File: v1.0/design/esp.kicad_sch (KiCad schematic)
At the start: 28 parts, among them J1 12402012E212A, J2 5v INPUT, J3 Conn_01x10, J4 Conn_01x10, SW1 PTS636_SM43_SMTR_LFS, SW2 PTS636_SM43_SMTR_LFS, U1 AMS1117-3.3, U1 ESP32-WROOM-E

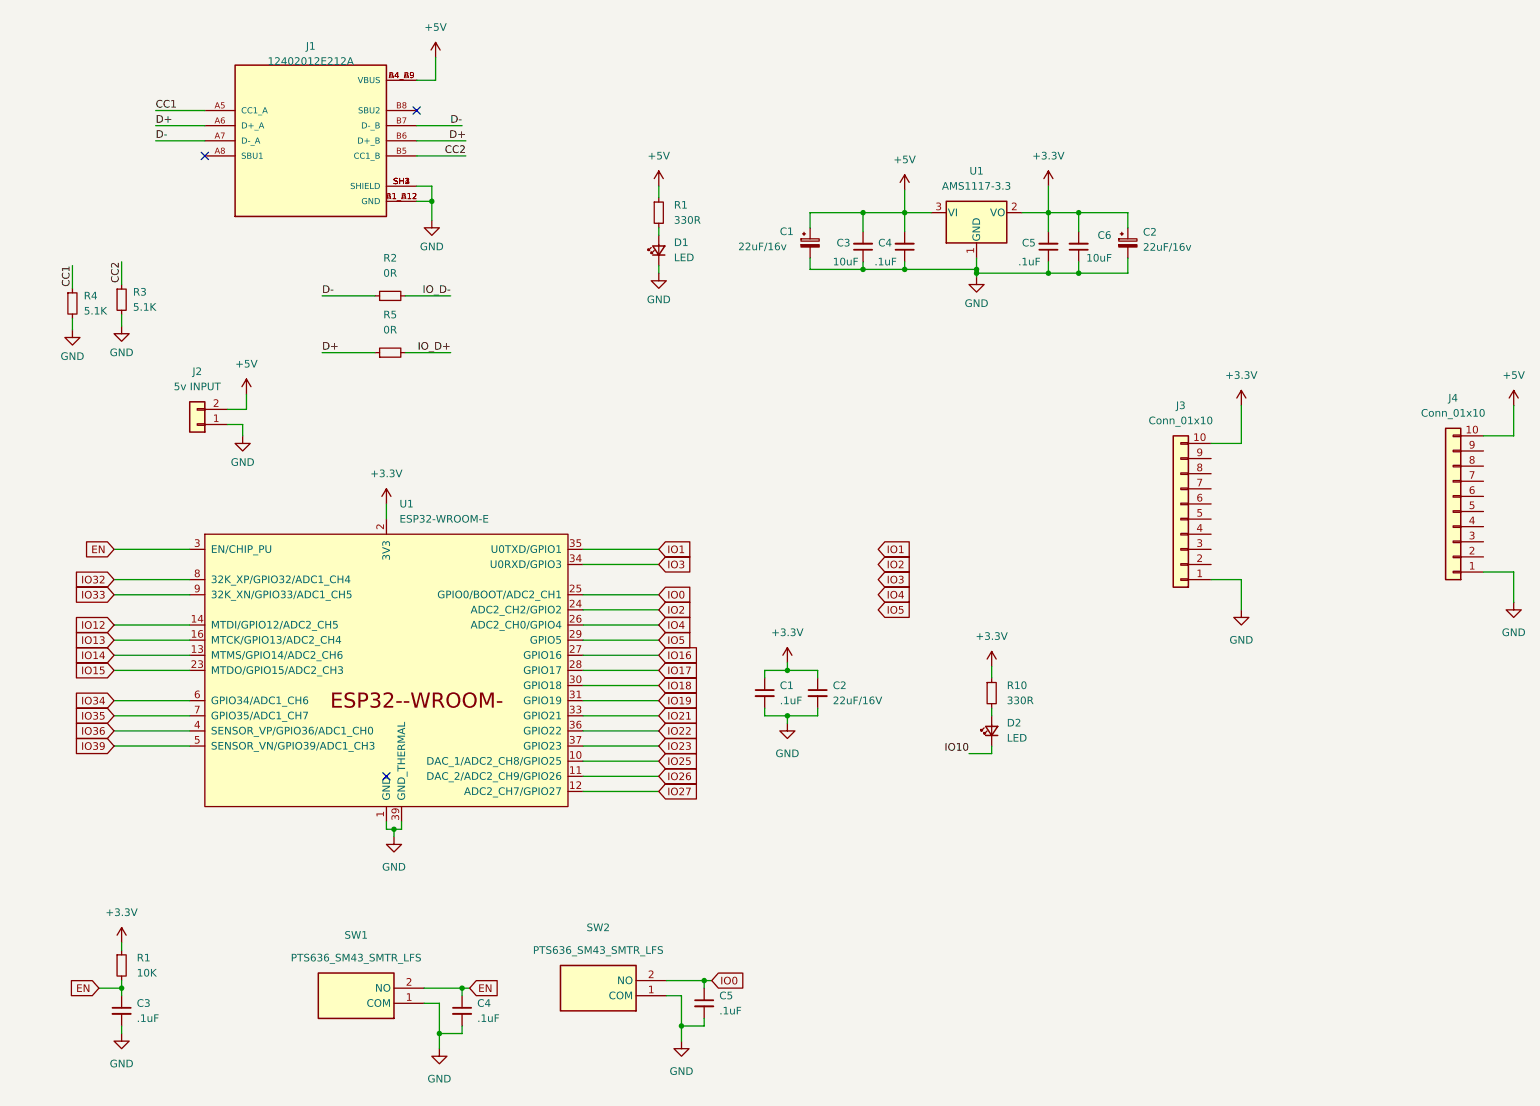
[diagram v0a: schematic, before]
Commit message: Schematic and pcb design is done
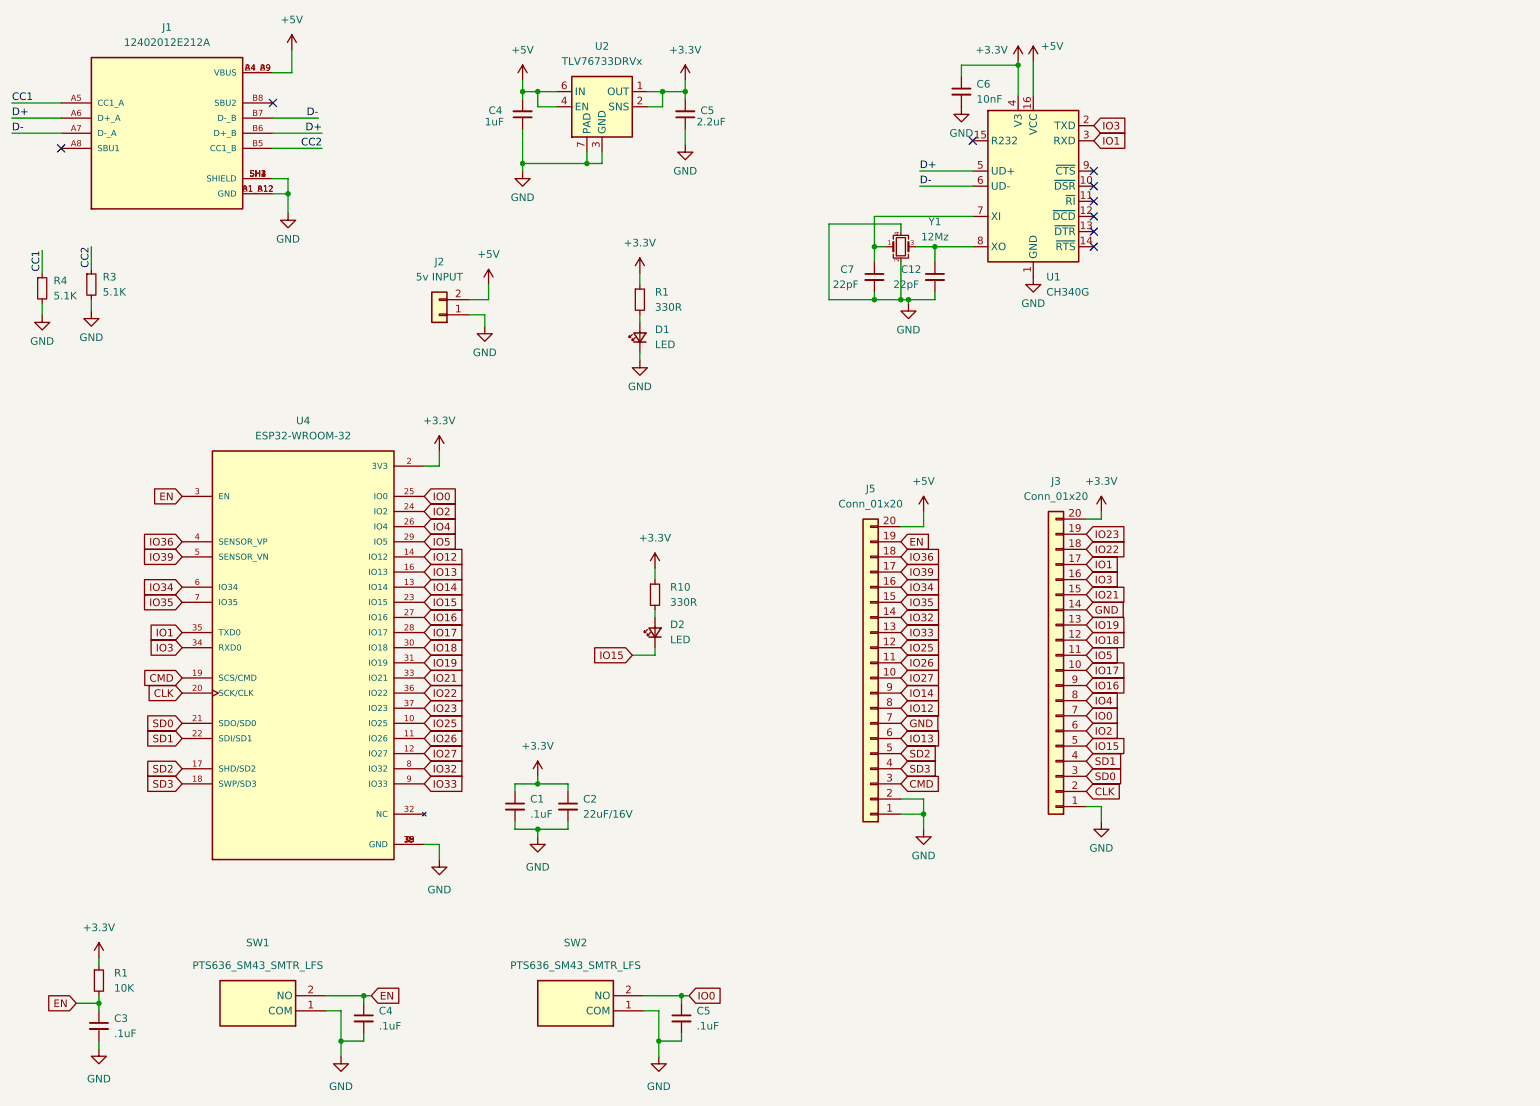
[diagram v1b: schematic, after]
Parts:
- removed C1, C2: 22uF/16v, Capacitor_Tantalum_SMD:CP_EIA-3216-10_Kemet-I, symbol Device:C_Polarized_Small
- removed C3: 10uF, Capacitor_SMD:C_0603_1608Metric, symbol Device:C_Small
- removed J3, J4: Conn_01x10, symbol Connector_Generic:Conn_01x10
- removed R2, R5: 0R, Resistor_SMD:R_0603_1608Metric, symbol Device:R_Small
- removed U1: AMS1117-3.3, Package_TO_SOT_SMD:SOT-223-3_TabPin2, symbol Regulator_Linear:AMS1117-3.3
- removed U1: ESP32-WROOM-E, Espressif:ESP32-WROOM-32E, symbol Espressif:ESP32-WROOM-E
- added C12, C7: 22pF, Capacitor_SMD:C_0603_1608Metric, symbol Device:C_Small
- added J3, J5: Conn_01x20, Connector_PinHeader_1.27mm:PinHeader_1x20_P1.27mm_Vertical, symbol Connector_Generic:Conn_01x20
- added U1: CH340G, Package_SO:SOIC-16_3.9x9.9mm_P1.27mm, symbol Interface_USB:CH340G
- added U2: TLV76733DRVx, Package_SON:WSON-6-1EP_2x2mm_P0.65mm_EP1x1.6mm_ThermalVias, symbol Regulator_Linear:TLV76733DRVx
- added U4: ESP32-WROOM-32, Footprint_KiCAD:ESP32-WROOM-32E, symbol ESP32-WROOM-32:ESP32-WROOM-32
- added Y1: 12Mz, Crystal:Crystal_SMD_Abracon_ABM10-4Pin_2.5x2.0mm, symbol Device:Crystal_GND24_Small
- C1, C2, C3, C4, C5: footprint (none) -> Capacitor_SMD:C_0603_1608Metric
- C4: value .1uF -> 1uF
- C5: value .1uF -> 2.2uF
- C6: value 10uF -> 10nF
- R1: footprint (none) -> Resistor_SMD:R_0603_1608Metric
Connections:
- net IO10 is gone; now on net IO15: D2.1 (K)
- net +3.3V: now also C6.1, R1.1, J3.20 (Pin_20), U1.4 (V3), U2.1 (OUT), U2.2 (SNS), U4.2 (3V3); no longer C6.2
- net +5V: now also J5.20 (Pin_20), U1.16 (VCC), U2.4 (EN), U2.6 (IN); no longer R1.1
- net D+: now also U1.5 (UD+)
- net D-: now also U1.6 (UD-)
- net EN: now also J5.19 (Pin_19), U4.3 (EN)
- net GND: now also C6.2, C12.2, C7.2, J3.1 (Pin_1), J3.14 (Pin_14), J5.1 (Pin_1), J5.2 (Pin_2), J5.7 (Pin_7), U1.1 (GND), U2.3 (GND), U2.5 (GND), U2.7 (PAD), U4.1 (GND), U4.15 (GND), U4.38 (GND), U4.39 (GND), Y1.2, Y1.4; no longer C6.1
- net IO0: now also J3.7 (Pin_7), U4.25 (IO0)
- net IO1: now also J3.17 (Pin_17), U1.3 (RXD), U4.35 (TXD0)
- net IO12: now also J5.8 (Pin_8), U4.14 (IO12)
- net IO13: now also J5.6 (Pin_6), U4.16 (IO13)
- net IO14: now also J5.9 (Pin_9), U4.13 (IO14)
- net IO15: now also J3.5 (Pin_5), U4.23 (IO15)
- net IO16: now also J3.9 (Pin_9), U4.27 (IO16)
- net IO17: now also J3.10 (Pin_10), U4.28 (IO17)
- net IO18: now also J3.12 (Pin_12), U4.30 (IO18)
- net IO19: now also J3.13 (Pin_13), U4.31 (IO19)
- net IO2: now also J3.6 (Pin_6), U4.24 (IO2)
- net IO21: now also J3.15 (Pin_15), U4.33 (IO21)
- net IO22: now also J3.18 (Pin_18), U4.36 (IO22)
- net IO23: now also J3.19 (Pin_19), U4.37 (IO23)
- net IO25: now also J5.12 (Pin_12), U4.10 (IO25)
- net IO26: now also J5.11 (Pin_11), U4.11 (IO26)
- net IO27: now also J5.10 (Pin_10), U4.12 (IO27)
- net IO3: now also J3.16 (Pin_16), U1.2 (TXD), U4.34 (RXD0)
- net IO32: now also J5.14 (Pin_14), U4.8 (IO32)
- net IO33: now also J5.13 (Pin_13), U4.9 (IO33)
- net IO34: now also J5.16 (Pin_16), U4.6 (IO34)
- net IO35: now also J5.15 (Pin_15), U4.7 (IO35)
- net IO36: now also J5.18 (Pin_18), U4.4 (SENSOR_VP)
- net IO39: now also J5.17 (Pin_17), U4.5 (SENSOR_VN)
- net IO4: now also J3.8 (Pin_8), U4.26 (IO4)
- net IO5: now also J3.11 (Pin_11), U4.29 (IO5)
- new net: C7.1, U1.7 (XI), Y1.1
- new net: C12.1, U1.8 (XO), Y1.3
- new net CLK: J3.2 (Pin_2), U4.20 (SCK/CLK)
- new net CMD: J5.3 (Pin_3), U4.19 (SCS/CMD)
- new net SD0: J3.3 (Pin_3), U4.21 (SDO/SD0)
- new net SD1: J3.4 (Pin_4), U4.22 (SDI/SD1)
- new net SD2: J5.5 (Pin_5), U4.17 (SHD/SD2)
- new net SD3: J5.4 (Pin_4), U4.18 (SWP/SD3)
- no-connect marks 3 -> 9
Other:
- moved on the sheet: C1, C2, C3, C4, C5, D1, D2, J2, R1, R10, R3, R4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
